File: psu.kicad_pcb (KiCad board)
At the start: 2 copper layers, 101.6 x 68.6 mm, 21 parts, among them J1 Conn_01x02_Socket, J2 Conn_01x03_Socket, U1 L7812, U2 L7912

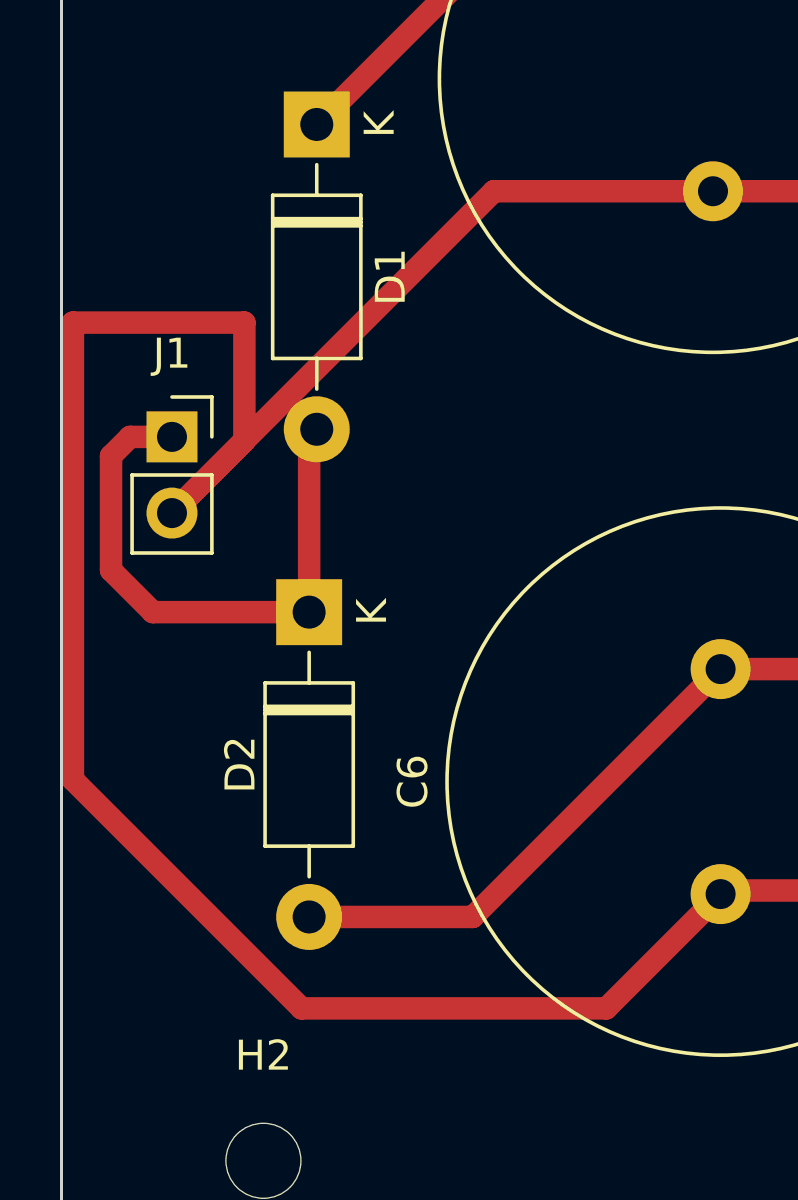
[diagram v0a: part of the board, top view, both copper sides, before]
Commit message: image
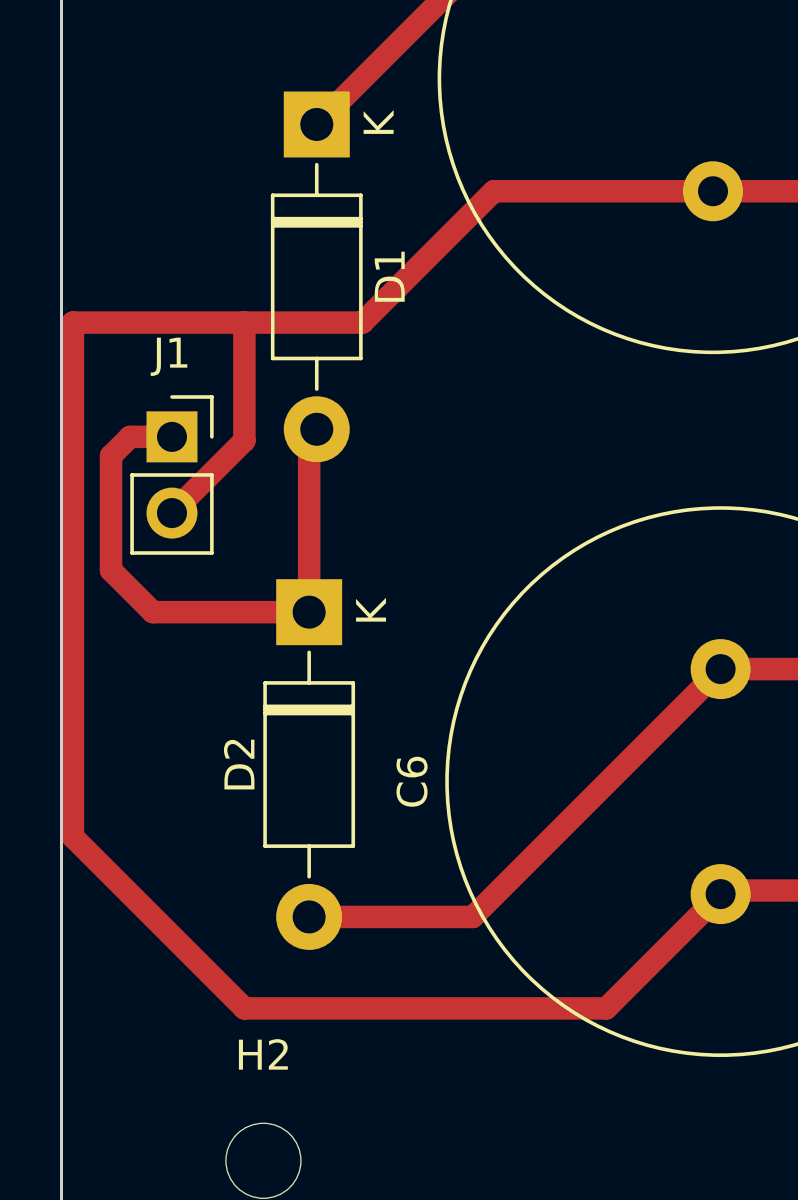
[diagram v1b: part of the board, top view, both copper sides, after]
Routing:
- net GND: track 225.4 -> 221.5 mm
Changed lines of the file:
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@@
   (segment (start 86.106 33.147) (end 89.408 33.147) (width 0.75) (layer "F.Cu") (net 1))
   (segment (start 89.408 33.147) (end 91.44 31.115) (width 0.75) (layer "F.Cu") (net 1))
+  (segment (start 22.352 45.085) (end 26.73 40.707) (width 0.75) (layer "F.Cu") (net 2))
+  (segment (start 18.415 45.085) (end 22.352 45.085) (width 0.75) (layer "F.Cu") (net 2))
   (segment (start 94.9255 40.647) (end 86.106 40.647) (width 0.75) (layer "F.Cu") (net 2))
-  (segment (start 18.415 45.085) (end 12.7 45.085) (width 0.75) (layer "F.Cu") (net 2))
-  (segment (start 30.48 67.945) (end 34.29 64.135) (width 0.75) (layer "F.Cu") (net 2))
+  (segment (start 12.7 45.085) (end 12.7 62.23) (width 0.75) (layer "F.Cu") (net 2))
+  (segment (start 16.002 51.435) (end 18.415 49.022) (width 0.75) (layer "F.Cu") (net 2))
   (segment (start 96.266 39.3065) (end 94.9255 40.647) (width 0.75) (layer "F.Cu") (net 2))
+  (segment (start 12.7 62.23) (end 18.415 67.945) (width 0.75) (layer "F.Cu") (net 2))
   (segment (start 85.986 40.767) (end 86.106 40.647) (width 0.75) (layer "F.Cu") (net 2))
   (segment (start 89.542 60.833) (end 86.36 64.015) (width 0.75) (layer "F.Cu") (net 2))
-  (segment (start 18.415 49.022) (end 18.415 45.085) (width 0.75) (layer "F.Cu") (net 2))
   (segment (start 91.694 60.833) (end 91.694 63.881) (width 0.75) (layer "F.Cu") (net 2))
   (segment (start 34.41 64.015) (end 34.29 64.135) (width 0.75) (layer "F.Cu") (net 2))
   (segment (start 72.898 40.767) (end 85.986 40.767) (width 0.75) (layer "F.Cu") (net 2))
-  (segment (start 12.7 60.325) (end 20.32 67.945) (width 0.75) (layer "F.Cu") (net 2))
   (segment (start 72.838 40.707) (end 72.898 40.767) (width 0.75) (layer "F.Cu") (net 2))
   (segment (start 110.49 45.085) (end 110.49 43.561) (width 0.75) (layer "F.Cu") (net 2))
   (segment (start 96.266 39.116) (end 96.266 37.719) (width 0.75) (layer "F.Cu") (net 2))
   (segment (start 110.49 43.561) (end 105.156 38.227) (width 0.75) (layer "F.Cu") (net 2))
+  (segment (start 30.48 67.945) (end 34.29 64.135) (width 0.75) (layer "F.Cu") (net 2))
+  (segment (start 18.415 49.022) (end 18.415 45.085) (width 0.75) (layer "F.Cu") (net 2))
   (segment (start 97.79 40.64) (end 96.266 39.116) (width 0.75) (layer "F.Cu") (net 2))
+  (segment (start 18.415 45.085) (end 12.7 45.085) (width 0.75) (layer "F.Cu") (net 2))
   (segment (start 91.694 60.833) (end 89.542 60.833) (width 0.75) (layer "F.Cu") (net 2))
-  (segment (start 12.7 45.085) (end 12.7 60.325) (width 0.75) (layer "F.Cu") (net 2))
   (segment (start 102.743 40.64) (end 97.79 40.64) (width 0.75) (layer "F.Cu") (net 2))
   (segment (start 96.266 37.719) (end 96.266 39.3065) (width 0.75) (layer "F.Cu") (net 2))
   (segment (start 105.156 38.227) (end 102.743 40.64) (width 0.75) (layer "F.Cu") (net 2))
   (segment (start 34.036 40.707) (end 53.848 40.707) (width 0.75) (layer "F.Cu") (net 2))
-  (segment (start 20.32 67.945) (end 30.48 67.945) (width 0.75) (layer "F.Cu") (net 2))
   (segment (start 86.36 64.015) (end 34.41 64.015) (width 0.75) (layer "F.Cu") (net 2))
   (segment (start 34.036 40.707) (end 26.73 40.707) (width 0.75) (layer "F.Cu") (net 2))
   (segment (start 91.694 63.881) (end 90.932 64.643) (width 0.75) (layer "F.Cu") (net 2))
-  (segment (start 26.73 40.707) (end 16.002 51.435) (width 0.75) (layer "F.Cu") (net 2))
   (segment (start 53.848 40.707) (end 72.838 40.707) (width 0.75) (layer "F.Cu") (net 2))
-  (segment (start 16.002 51.435) (end 18.415 49.022) (width 0.75) (layer "F.Cu") (net 2))
+  (segment (start 18.415 67.945) (end 30.48 67.945) (width 0.75) (layer "F.Cu") (net 2))
   (segment (start 34.29 56.635) (end 53.594 56.635) (width 0.75) (layer "F.Cu") (net 3))
   (segment (start 86.24 56.635) (end 86.36 56.515) (width 0.75) (layer "F.Cu") (net 3))
